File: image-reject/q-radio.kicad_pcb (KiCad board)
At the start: 6 copper layers, 120 x 75 mm, 25 parts, among them U1 MXD8546F, U9 MXD8638C

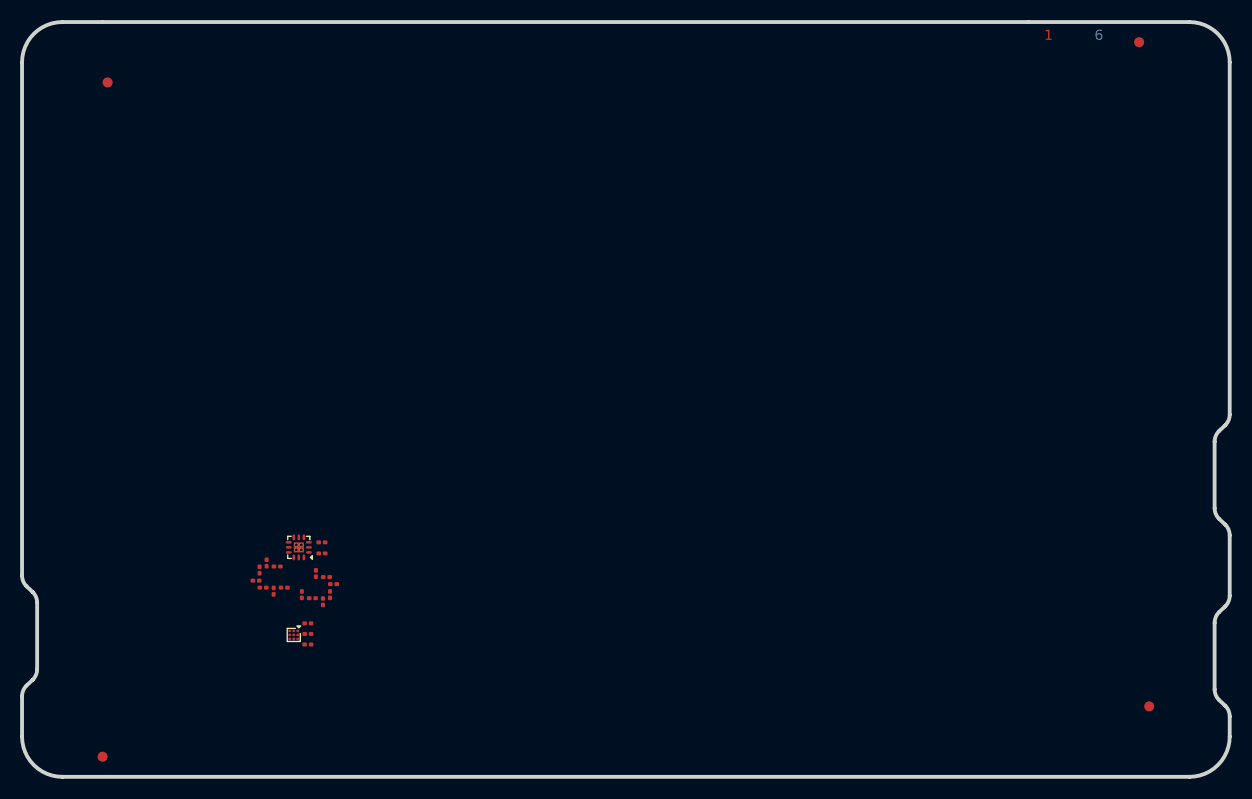
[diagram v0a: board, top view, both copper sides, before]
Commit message: All sub-modules added to child projects
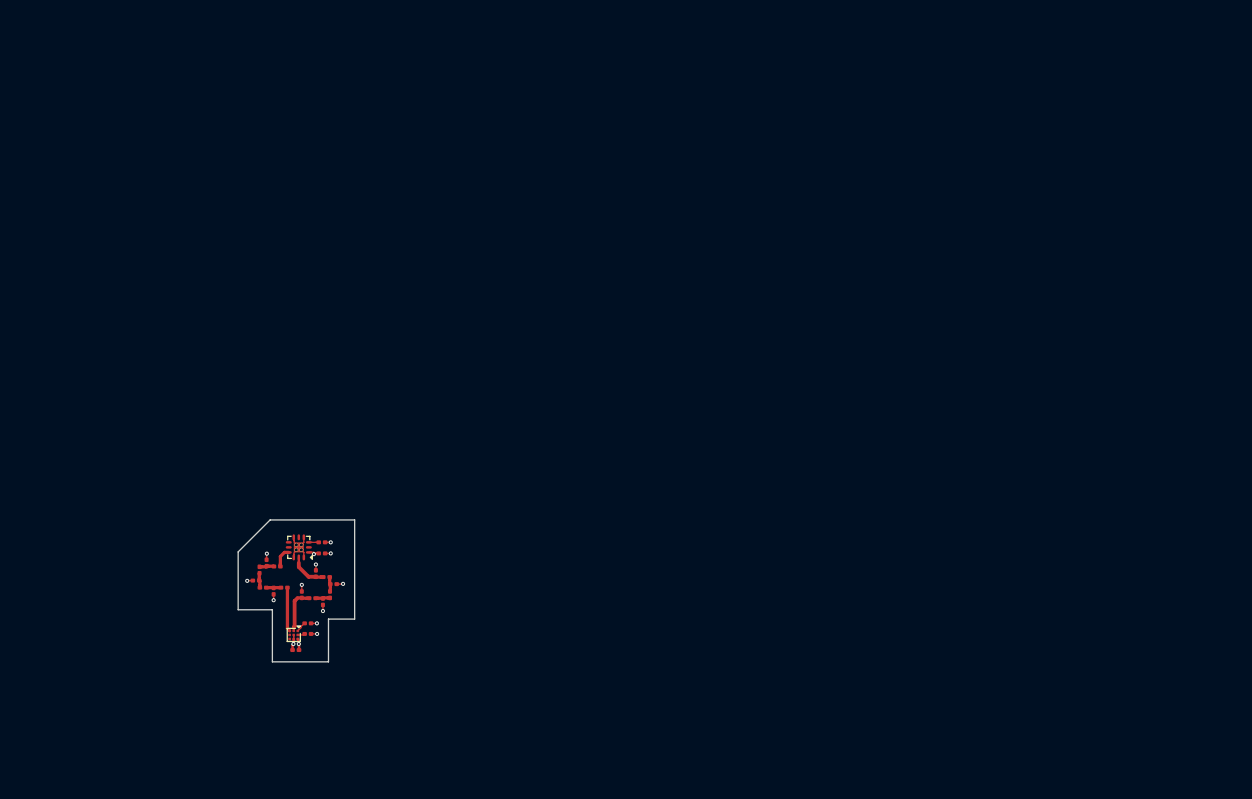
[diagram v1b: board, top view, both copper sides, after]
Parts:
- removed FID1, FID2, FID3, FID4: Fiducial_1mm_Mask2mm, Fiducial:Fiducial_1mm_Mask2mm
- moved C31 1.32 mm to (87.2, 162.4), turned to 180 degrees
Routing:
- net GND: track 0.00 -> 12.1 mm, vias 0 -> 12
- net Net-(U9-RF3): track 0.00 -> 4.59 mm
- net Net-(U9-RF1): track 0.00 -> 4.38 mm
- net Net-(U1-RF3): track 0.00 -> 3.99 mm
- net 2V5RF: track 0.00 -> 3.43 mm, vias 0 -> 2
- net Net-(U1-RF4): track 0.00 -> 2.27 mm
- net Net-(C103-Pad2): track 0.00 -> 1.48 mm
- net Net-(C54-Pad1): track 0.00 -> 1.47 mm
- net Net-(C101-Pad1): track 0.00 -> 1.47 mm
- net Net-(C56-Pad1): track 0.00 -> 1.47 mm
- net Net-(C101-Pad2): track 0.00 -> 1.47 mm
- net /Image Reject Filters/MIX_EN: track 0.00 -> 1.05 mm
- net /Image Reject Filters/RX_XOR_LPF: track 0.00 -> 0.98 mm
- net /Image Reject Filters/LPF_OR_MIX_BYPASS: track 0.00 -> 0.72 mm
- added copper zone on In2.Cu, net 2V5RF
- added copper zone on In1.Cu, net GND
- added copper zone on In4.Cu, net GND
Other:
- board size 120 x 75 mm -> 11.6 x 14.1 mm
- board text removed: "1"
- board text removed: "2"
- board text removed: "3"
- board text removed: "4"
- board text removed: "5"
- board text removed: "6"
